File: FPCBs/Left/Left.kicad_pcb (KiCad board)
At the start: 2 copper layers, 46.9 x 13.4 mm, 7 parts, among them J1 To PCB, SW1 SW_Rotary_1x6_MP

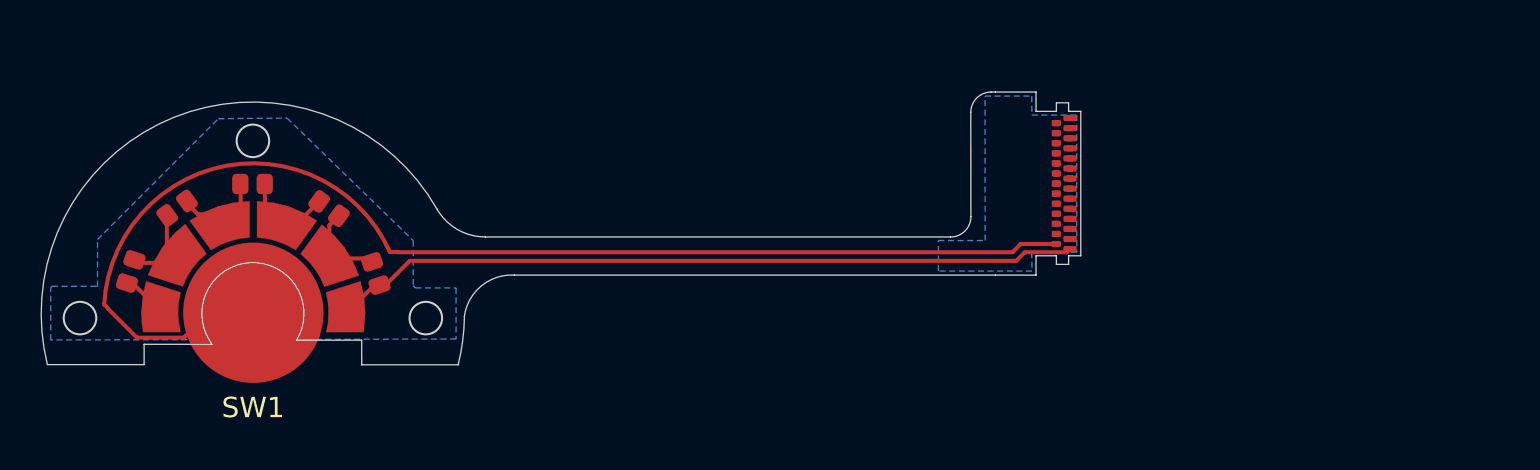
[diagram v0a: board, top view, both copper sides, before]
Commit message: Fix left fpcb
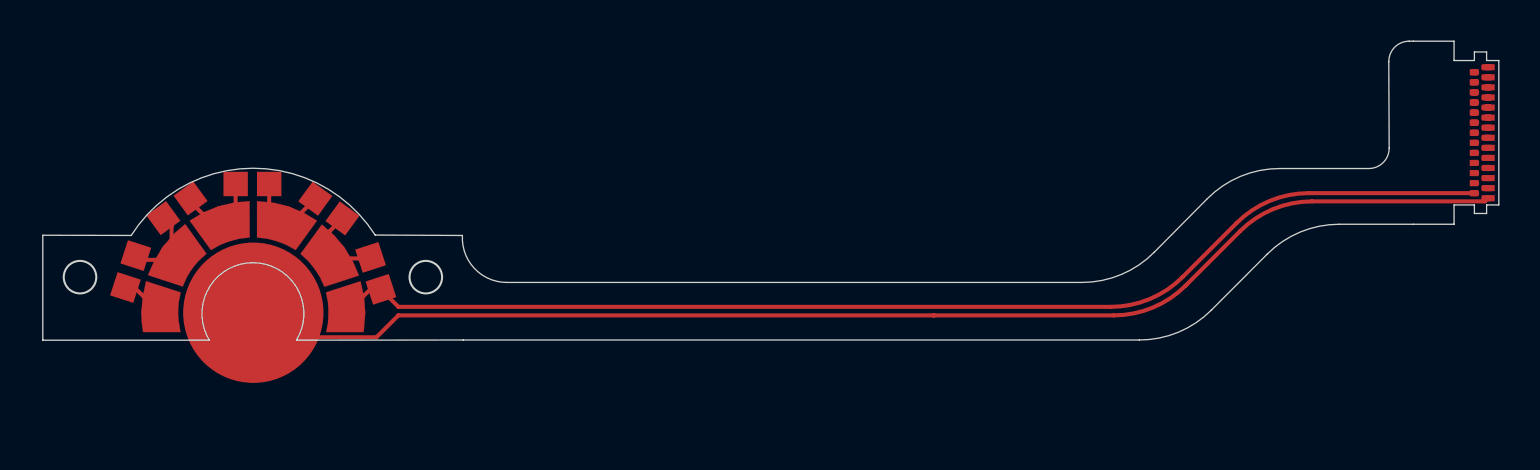
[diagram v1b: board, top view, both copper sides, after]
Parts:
- R1: value 1.8K -> 1.7K; footprint Leica-G9ii:R_2x1mm -> Leica-G9ii:R_0603
- R2: value 2.8K -> 2.7K; footprint Leica-G9ii:R_2x1mm -> Leica-G9ii:R_0603
- R3: value 4.8K -> 4.7K; footprint Leica-G9ii:R_2x1mm -> Leica-G9ii:R_0603
- R4: value 8K -> 8.2K; footprint Leica-G9ii:R_2x1mm -> Leica-G9ii:R_0603
- R5: value R -> 22K; footprint Leica-G9ii:R_2x1mm -> Leica-G9ii:R_0603
- moved J1 20.7 mm to (167.6, 91.1)
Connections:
- R1 pad 1: Net-(J1-Pin_1) -> Net-(J1-Pin_2)
- SW1 pad 1: Net-(J1-Pin_1) -> Net-(J1-Pin_2)
- SW1 pad 7: Net-(J1-Pin_2) -> Net-(J1-Pin_1)
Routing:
- net Net-(J1-Pin_1): track 36.9 -> 68.8 mm
- net Net-(J1-Pin_2): track 49.0 -> 58.1 mm
- net Net-(R4-Pad2): track 4.97 -> 4.41 mm
- removed copper zone on B.Cu, net (none)
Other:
- board size 46.9 x 13.4 mm -> 67.4 x 14.7 mm
